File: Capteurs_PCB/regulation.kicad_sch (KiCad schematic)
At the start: 12 parts, among them U4 RS PRO 1W isolated DC-DC conv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, U5 RS PRO 1W isolated DC-DC conv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

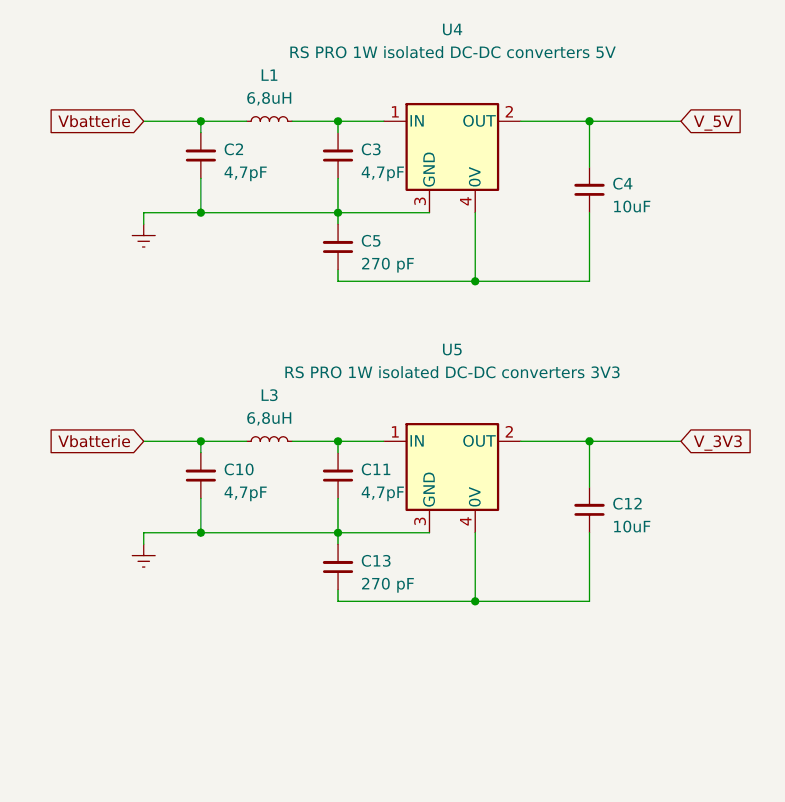
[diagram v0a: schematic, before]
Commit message: pcb update
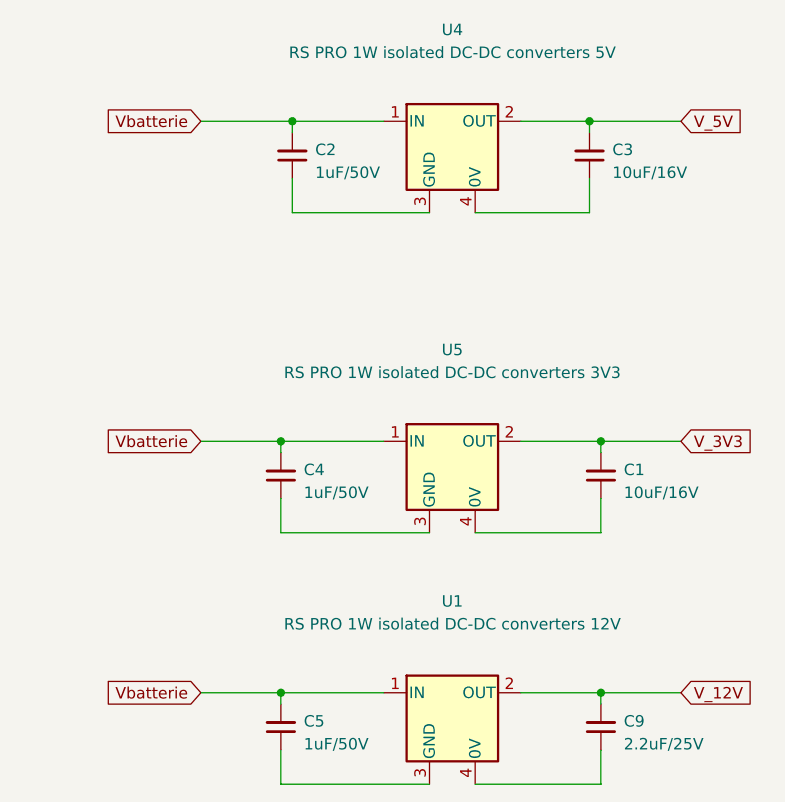
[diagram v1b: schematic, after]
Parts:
- removed C10, C11: 4,7pF, symbol Device:C_Small
- removed C13: 270 pF, symbol Device:C_Small
- removed L1, L3: 6,8uH, symbol Device:L_Small
- added C9: 2.2uF/25V, symbol Device:C_Small
- added U1: RS PRO 1W isolated DC-DC converters 12V, Package_TO_SOT_THT:TO-220-4_Vertical, symbol Regulator_Linear:KA378R05
- C1: renamed from C12; value 10uF -> 10uF/16V
- C2: value 4,7pF -> 1uF/50V
- C3: value 4,7pF -> 10uF/16V
- C4: value 10uF -> 1uF/50V
- C5: value 270 pF -> 1uF/50V
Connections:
- net V_5V: now also C3.2; no longer C4.2
- net Vbatterie: now also C4.2, C5.2, U4.1 (IN), U5.1 (IN), U1.1 (IN)
- removed net Earth: C2.1, C3.1, C5.2, U4.3 (GND), U5.3 (GND)
- new net: C3.1, U4.4 (0V)
- new net: C2.1, U4.3 (GND)
- new net: C4.1, U5.3 (GND)
- new net: C5.1, U1.3 (GND)
- new net: C9.1, U1.4 (0V)
- new net V_12V: C9.2, U1.2 (OUT)
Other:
- moved on the sheet: C1
